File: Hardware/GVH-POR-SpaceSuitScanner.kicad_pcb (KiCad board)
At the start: 2 copper layers, 68.1 x 221.9 mm, 49 parts, among them J1 Phoenix _725656, J10 Phoenix_5POS_1725685, J11 Phoenix _725656, J12 Phoenix _725656, J13 Phoenix _725656, J14 Phoenix _725656, J15 Phoenix _725656, J16 Phoenix _725656, J17 Phoenix _725656, J18 Phoenix _725656, J19 Phoenix_3POS_1725669, J2 Phoenix _725656, J29 n00d i2c, J3 Phoenix _725656, J30 Matrix i2c, J31 Speaker In, J32 Speaker, J4 Phoenix _725656, J5 Phoenix _725656, J6 Phoenix _725656, J7 Phoenix _725656, J8 Phoenix _725656, J9 Phoenix _725656, U1 AW9523, U2 AW9523, U3 AW9523 Expander, U4 AW9523 Expander, U5 AT42QT1010, U6 IS31FL3731 LED Driver

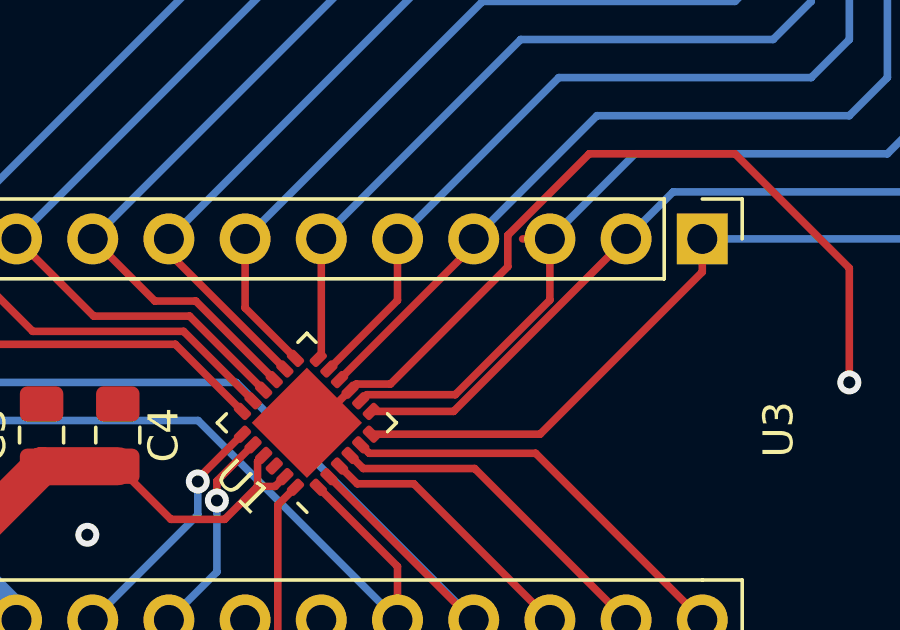
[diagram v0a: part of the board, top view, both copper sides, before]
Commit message: Backing up again
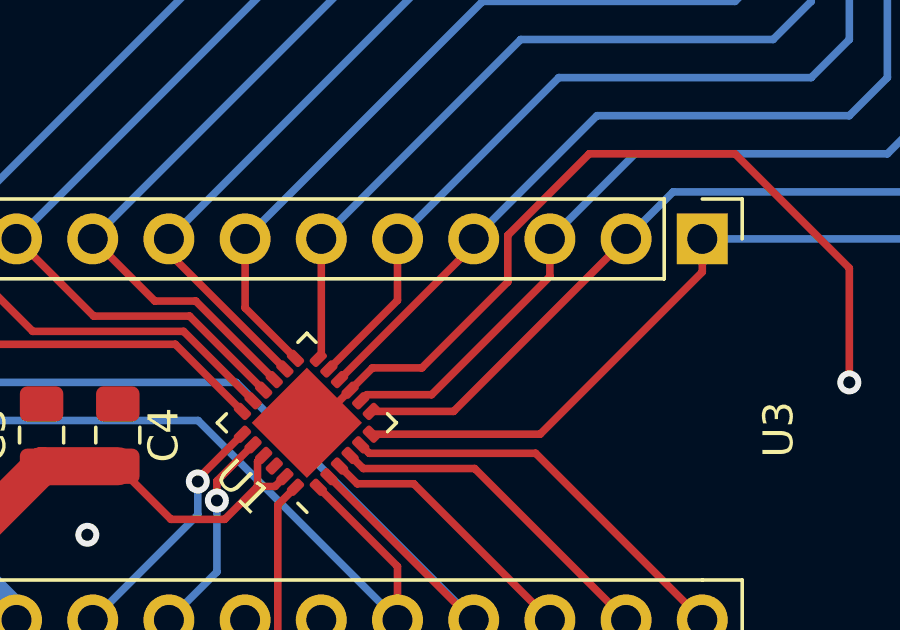
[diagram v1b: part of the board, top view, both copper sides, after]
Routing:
- net P01_3: track 176.2 -> 174.9 mm
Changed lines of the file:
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@@
   (segment (start 88.138 181.229) (end 89.535 182.626) (width 0.254) (layer "B.Cu") (net 1))
   (segment (start 97.79 175.26) (end 99.06 173.99) (width 0.254) (layer "F.Cu") (net 2))
-  (segment (start 99.106068 153.623932) (end 99.106068 152.576953) (width 0.254) (layer "F.Cu") (net 2))
   (segment (start 92.409 179.5272) (end 92.762553 179.5272) (width 0.254) (layer "F.Cu") (net 2))
   (segment (start 92.02893 160.974967) (end 91.44 161.563897) (width 0.254) (layer "F.Cu") (net 2))
   (segment (start 97.029753 175.26) (end 97.79 175.26) (width 0.254) (layer "F.Cu") (net 2))
-  (segment (start 99.106068 152.576953) (end 101.823021 149.86) (width 0.254) (layer "F.Cu") (net 2))
   (segment (start 110.49 153.67) (end 110.49 157.48) (width 0.254) (layer "F.Cu") (net 2))
   (segment (start 78.74 156.21) (end 74.93 160.02) (width 0.254) (layer "F.Cu") (net 2))
@@
   (segment (start 81.28 156.21) (end 78.74 156.21) (width 0.254) (layer "F.Cu") (net 2))
   (segment (start 93.84973 178.440023) (end 97.029753 175.26) (width 0.254) (layer "F.Cu") (net 2))
-  (segment (start 94.053469 157.536214) (end 95.193786 157.536214) (width 0.254) (layer "F.Cu") (net 2))
   (segment (start 90.261163 158.44706) (end 88.024103 156.21) (width 0.254) (layer "F.Cu") (net 2))
-  (segment (start 93.84973 157.739953) (end 94.053469 157.536214) (width 0.254) (layer "F.Cu") (net 2))
+  (segment (start 101.823021 149.86) (end 106.68 149.86) (width 0.254) (layer "F.Cu") (net 2))
   (segment (start 82.729 185.8772) (end 82.729 187.781) (width 1.27) (layer "F.Cu") (net 2))
   (segment (start 92.02893 181.675037) (end 91.44 182.263967) (width 0.254) (layer "F.Cu") (net 2))
@@
   (segment (start 82.729 187.781) (end 81.28 189.23) (width 1.27) (layer "F.Cu") (net 2))
   (segment (start 92.762553 158.82713) (end 93.84973 157.739953) (width 0.254) (layer "F.Cu") (net 2))
-  (segment (start 101.823021 149.86) (end 106.68 149.86) (width 0.254) (layer "F.Cu") (net 2))
   (segment (start 99.06 173.99) (end 99.06 168.91) (width 0.254) (layer "F.Cu") (net 2))
-  (segment (start 106.68 149.86) (end 110.49 153.67) (width 0.254) (layer "F.Cu") (net 2))
+  (segment (start 96.2406 156.9974) (end 99.106068 154.131932) (width 0.254) (layer "F.Cu") (net 2))
   (segment (start 92.762553 179.5272) (end 93.84973 178.440023) (width 0.254) (layer "F.Cu") (net 2))
   (segment (start 91.44 161.563897) (end 91.44 170.18) (width 0.254) (layer "F.Cu") (net 2))
-  (segment (start 95.193786 157.536214) (end 99.106068 153.623932) (width 0.254) (layer "F.Cu") (net 2))
+  (segment (start 106.68 149.86) (end 110.49 153.67) (width 0.254) (layer "F.Cu") (net 2))
+  (segment (start 94.592283 156.9974) (end 96.2406 156.9974) (width 0.254) (layer "F.Cu") (net 2))
+  (segment (start 99.106068 152.576953) (end 101.823021 149.86) (width 0.254) (layer "F.Cu") (net 2))
+  (segment (start 99.106068 154.131932) (end 99.106068 152.576953) (width 0.254) (layer "F.Cu") (net 2))
+  (segment (start 93.84973 157.739953) (end 94.592283 156.9974) (width 0.254) (layer "F.Cu") (net 2))
   (via (at 67.31 152.4) (size 0.8) (drill 0.4) (layers "F.Cu" "B.Cu") (net 2))
   (via (at 85.09 162.56) (size 0.8) (drill 0.4) (layers "F.Cu" "B.Cu") (free) (net 2))
@@
   (segment (start 104.61613 151.13) (end 113.03 151.13) (width 0.254) (layer "B.Cu") (net 17))
   (segment (start 103.049 152.69713) (end 104.61613 151.13) (width 0.254) (layer "B.Cu") (net 17))
-  (segment (start 94.406576 157.890214) (end 97.355284 157.890214) (width 0.254) (layer "F.Cu") (net 18))
+  (segment (start 96.566986 157.890214) (end 100.509 153.9482) (width 0.254) (layer "F.Cu") (net 18))
+  (segment (start 100.509 153.9482) (end 100.509 152.69713) (width 0.254) (layer "F.Cu") (net 18))
   (segment (start 94.203283 158.093507) (end 94.406576 157.890214) (width 0.254) (layer "F.Cu") (net 18))
-  (segment (start 100.509 154.736498) (end 100.509 152.69713) (width 0.254) (layer "F.Cu") (net 18))
-  (segment (start 100.509 152.69713) (end 99.59966 152.69713) (width 0.254) (layer "F.Cu") (net 18))
-  (segment (start 97.355284 157.890214) (end 100.509 154.736498) (width 0.254) (layer "F.Cu") (net 18))
+  (segment (start 94.406576 157.890214) (end 96.566986 157.890214) (width 0.254) (layer "F.Cu") (net 18))
   (segment (start 105.8672 49.9872) (end 56.059 49.9872) (width 0.254) (layer "B.Cu") (net 18))
   (segment (start 100.509 152.69713) (end 103.34613 149.86) (width 0.254) (layer "B.Cu") (net 18))
